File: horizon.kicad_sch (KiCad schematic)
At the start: 40 parts, among them J2 Conn_02x03_Counter_Clockwise, J7 Conn_02x03_Counter_Clockwise, J8 Conn_02x03_Counter_Clockwise, U1 MMCU, U3 NMCU, U4 TMCU, Y1 Crystal

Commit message: footprints
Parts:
- C10, C11, C9: footprint (none) -> Capacitor_SMD:C_0603_1608Metric
- C12, C13, C17, C61, C62, C63, C64, C65, C66, C67, C68, C69, C70, C71, C72, C73, C74, C75, C76, C77, C78: footprint (none) -> Capacitor_SMD:C_0201_0603Metric
- R26, R28, R29, R3, R30, R4, R5, R6, R7: footprint (none) -> Resistor_SMD:R_0603_1608Metric
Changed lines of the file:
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@@
 			)
 		)
-		(property "Footprint" ""
+		(property "Footprint" "Resistor_SMD:R_0603_1608Metric"
 			(at 31.242 175.26 90)
 			(effects
@@
 			)
 		)
-		(property "Footprint" ""
+		(property "Footprint" "Capacitor_SMD:C_0201_0603Metric"
 			(at 148.59 54.9148 0)
 			(effects
@@
 			)
 		)
-		(property "Footprint" ""
+		(property "Footprint" "Resistor_SMD:R_0603_1608Metric"
 			(at 176.022 76.2 90)
 			(effects
@@
 			)
 		)
-		(property "Footprint" ""
+		(property "Footprint" "Capacitor_SMD:C_0201_0603Metric"
 			(at 148.59 53.0352 0)
 			(effects
@@
 			)
 		)
-		(property "Footprint" ""
+		(property "Footprint" "Resistor_SMD:R_0603_1608Metric"
 			(at 248.412 170.18 90)
 			(effects
@@
 			)
 		)
-		(property "Footprint" ""
+		(property "Footprint" "Capacitor_SMD:C_0201_0603Metric"
 			(at 281.6352 77.47 0)
 			(effects
@@
 			)
 		)
-		(property "Footprint" ""
+		(property "Footprint" "Capacitor_SMD:C_0201_0603Metric"
 			(at 148.59 49.8348 0)
 			(effects
@@
 			)
 		)
-		(property "Footprint" ""
+		(property "Footprint" "Capacitor_SMD:C_0201_0603Metric"
 			(at 148.59 58.1152 0)
 			(effects
@@
 			)
 		)
-		(property "Footprint" ""
+		(property "Footprint" "Resistor_SMD:R_0603_1608Metric"
 			(at 107.442 109.22 90)
 			(effects
@@
 			)
 		)
-		(property "Footprint" ""
+		(property "Footprint" "Capacitor_SMD:C_0201_0603Metric"
 			(at 43.18 54.9148 0)
 			(effects
@@
 			)
 		)
-		(property "Footprint" ""
+		(property "Footprint" "Resistor_SMD:R_0603_1608Metric"
 			(at 201.422 96.52 90)
 			(effects
@@
 			)
 		)
-		(property "Footprint" ""
+		(property "Footprint" "Capacitor_SMD:C_0201_0603Metric"
 			(at 280.9748 44.45 0)
 			(effects
@@
 			)
 		)
-		(property "Footprint" ""
+		(property "Footprint" "Capacitor_SMD:C_0201_0603Metric"
 			(at 341.9348 39.37 0)
 			(effects
@@
 			)
 		)
-		(property "Footprint" ""
+		(property "Footprint" "Capacitor_SMD:C_0603_1608Metric"
 			(at 294.64 109.5248 0)
 			(effects
@@
 			)
 		)
-		(property "Footprint" ""
+		(property "Footprint" "Resistor_SMD:R_0603_1608Metric"
 			(at 136.652 181.61 90)
 			(effects
@@
 			)
 		)
-		(property "Footprint" ""
+		(property "Footprint" "Capacitor_SMD:C_0201_0603Metric"
 			(at 53.34 46.0248 0)
 			(effects
@@
 			)
 		)
-		(property "Footprint" ""
+		(property "Footprint" "Capacitor_SMD:C_0201_0603Metric"
 			(at 288.29 103.1748 0)
 			(effects
@@
 			)
 		)
-		(property "Footprint" ""
+		(property "Footprint" "Capacitor_SMD:C_0201_0603Metric"
 			(at 288.29 53.6448 0)
 			(effects
@@
 			)
 		)
-		(property "Footprint" ""
+		(property "Footprint" "Capacitor_SMD:C_0201_0603Metric"
 			(at 53.34 54.3052 0)
 			(effects
@@
 			)
 		)
-		(property "Footprint" ""
+		(property "Footprint" "Capacitor_SMD:C_0201_0603Metric"
 			(at 345.1352 57.15 0)
 			(effects
@@
 			)
 		)
-		(property "Footprint" ""
+		(property "Footprint" "Capacitor_SMD:C_0201_0603Metric"
 			(at 53.34 49.2252 0)
 			(effects
@@
 			)
 		)
-		(property "Footprint" ""
+		(property "Footprint" "Capacitor_SMD:C_0201_0603Metric"
 			(at 53.34 51.1048 0)
 			(effects
@@
 			)
 		)
-		(property "Footprint" ""
+		(property "Footprint" "Capacitor_SMD:C_0201_0603Metric"
 			(at 148.59 157.1752 0)
 			(effects
@@
 			)
 		)
-		(property "Footprint" ""
+		(property "Footprint" "Capacitor_SMD:C_0201_0603Metric"
 			(at 294.64 117.1448 0)
 			(effects
@@
 			)
 		)
-		(property "Footprint" ""
+		(property "Footprint" "Capacitor_SMD:C_0603_1608Metric"
 			(at 341.3252 62.23 0)
 			(effects
@@
 			)
 		)
-		(property "Footprint" ""
+		(property "Footprint" "Resistor_SMD:R_0603_1608Metric"
 			(at 216.408 114.3 90)
 			(effects
@@
 			)
 		)
-		(property "Footprint" ""
+		(property "Footprint" "Capacitor_SMD:C_0201_0603Metric"
 			(at 138.43 58.7248 0)
 			(effects
@@
 			)
 		)
-		(property "Footprint" ""
+		(property "Footprint" "Capacitor_SMD:C_0201_0603Metric"
 			(at 53.34 44.1452 0)
 			(effects
@@
 			)
 		)
-		(property "Footprint" ""
+		(property "Footprint" "Resistor_SMD:R_0603_1608Metric"
 			(at 198.882 124.46 90)
 			(effects
@@
 			)
 		)
-		(property "Footprint" ""
+		(property "Footprint" "Capacitor_SMD:C_0201_0603Metric"
 			(at 281.6352 67.31 0)
 			(effects
@@
 			)
 		)
-		(property "Footprint" ""
+		(property "Footprint" "Resistor_SMD:R_0603_1608Metric"
 			(at 192.532 127 90)
 			(effects
@@
 			)
 		)
-		(property "Footprint" ""
+		(property "Footprint" "Capacitor_SMD:C_0201_0603Metric"
 			(at 148.59 47.9552 0)
 			(effects
@@
 			)
 		)
-		(property "Footprint" ""
+		(property "Footprint" "Capacitor_SMD:C_0603_1608Metric"
 			(at 341.3252 72.39 0)
 			(effects

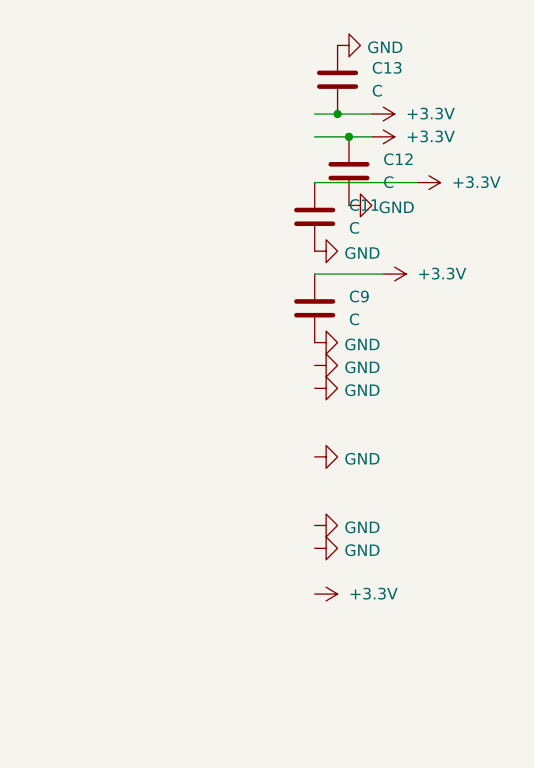
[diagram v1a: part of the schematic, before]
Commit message: clean up
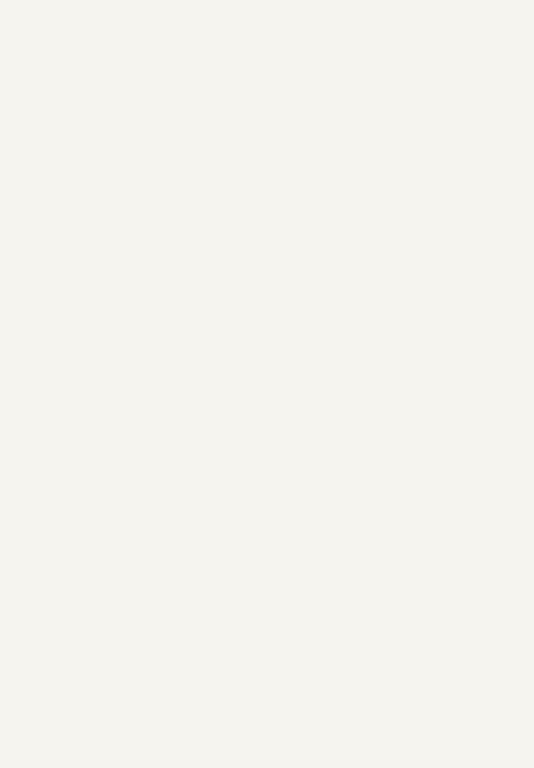
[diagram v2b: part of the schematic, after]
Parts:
- removed C11, C9: C, Capacitor_SMD:C_0603_1608Metric, symbol Device:C
- removed C12, C13: C, Capacitor_SMD:C_0201_0603Metric, symbol Device:C
